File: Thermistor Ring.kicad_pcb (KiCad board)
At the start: 2 copper layers, 70 x 70 mm, 20 parts, among them IC1 MAX30210ENL+, IC2 MAX30210ENL+, IC3 MAX30210ENL+, IC4 MAX30210ENL+, IC5 MAX30210ENL+, IC6 MAX30210ENL+, J1 Conn_01x04_Socket, J3 Conn_01x03_Socket, U1 TPS7A2018PDBVR

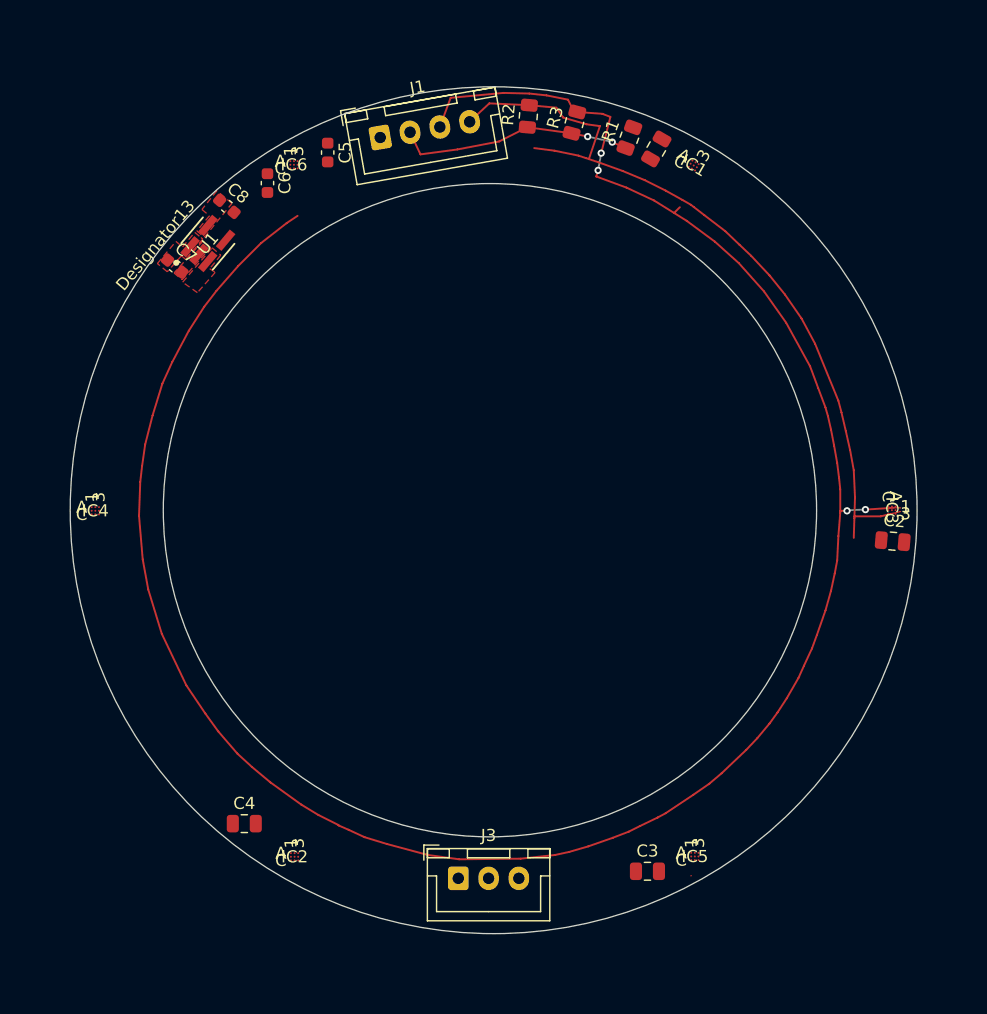
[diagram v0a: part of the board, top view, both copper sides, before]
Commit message: v0.1 alpha for review
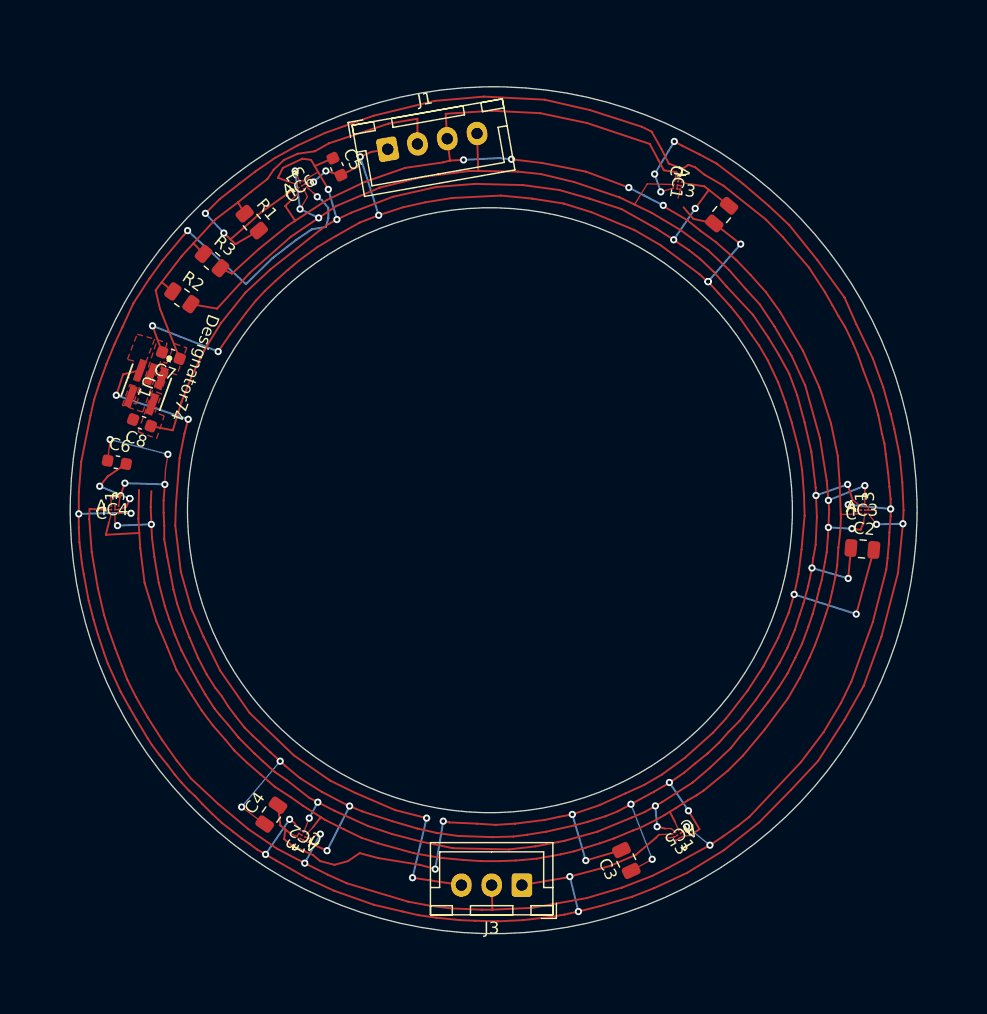
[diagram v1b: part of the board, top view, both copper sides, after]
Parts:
- U1: footprint LDO_TSA7A:DBV0005A-IPC_A -> TPS7A201:DBV0005A-IPC_A
- moved R2 32.3 mm to (188.1, 53.6), turned to -35 degrees
- moved R3 32.1 mm to (190.6, 50.5), turned to -40 degrees
- moved R1 32.0 mm to (193.9, 47.3), turned to -50 degrees
- moved C6 26.2 mm to (182.8, 67.2), turned to -10 degrees
- moved C8 19.2 mm to (184.8, 63.9), turned to 160 degrees
- moved U1 12.9 mm to (185.2, 61.0), turned to -110 degrees
- moved C1 7.66 mm to (232.8, 46.7), turned to -130 degrees
- moved C7 7.40 mm to (187.2, 58.3), turned to 160 degrees
- moved J3 5.28 mm to (216.3, 102.1), turned to 180 degrees
- moved C2 2.59 mm to (244.4, 74.3)
- moved C4 2.36 mm to (195.5, 96.3), turned to 55 degrees
- moved IC5 2.27 mm to (229.1, 98.0), turned to -150 degrees
- moved IC3 2.24 mm to (244.6, 71.1), turned to 0 degrees
- moved IC1 2.11 mm to (229.1, 44.3), turned to -100 degrees
- moved C3 1.96 mm to (224.9, 100.1), turned to 115 degrees
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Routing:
- net /VDD: track 0.00 -> 244.5 mm, vias 0 -> 20
- net /CVT/PDB: track 0.00 -> 224.6 mm, vias 0 -> 13
- net /INT: track 0.00 -> 213.3 mm, vias 0 -> 8
- net GND: track 0.00 -> 195.9 mm, vias 0 -> 18
- net /SCL: track 64.7 -> 196.8 mm, vias 0 -> 13
- net /ENABLE: track 0.00 -> 61.8 mm, vias 0 -> 4
- net /Power 3.3-5V: track 19.6 -> 38.4 mm, vias 2 -> 0
- net /SDA: track 183.6 -> 202.3 mm
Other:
- outline, holes or cut-outs redrawn

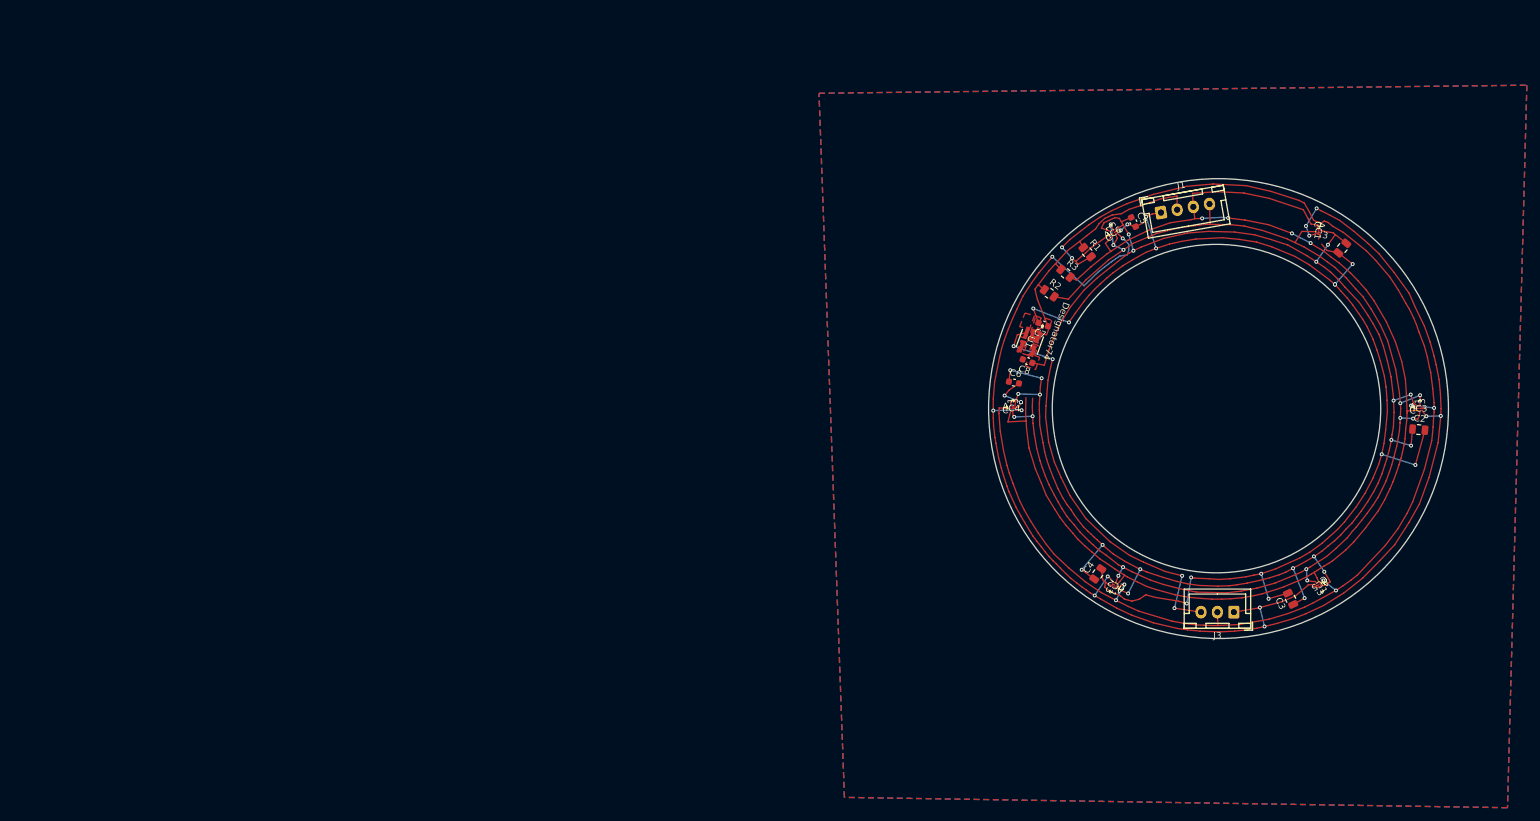
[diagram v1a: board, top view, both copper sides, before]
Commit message: changing to smaller diameter
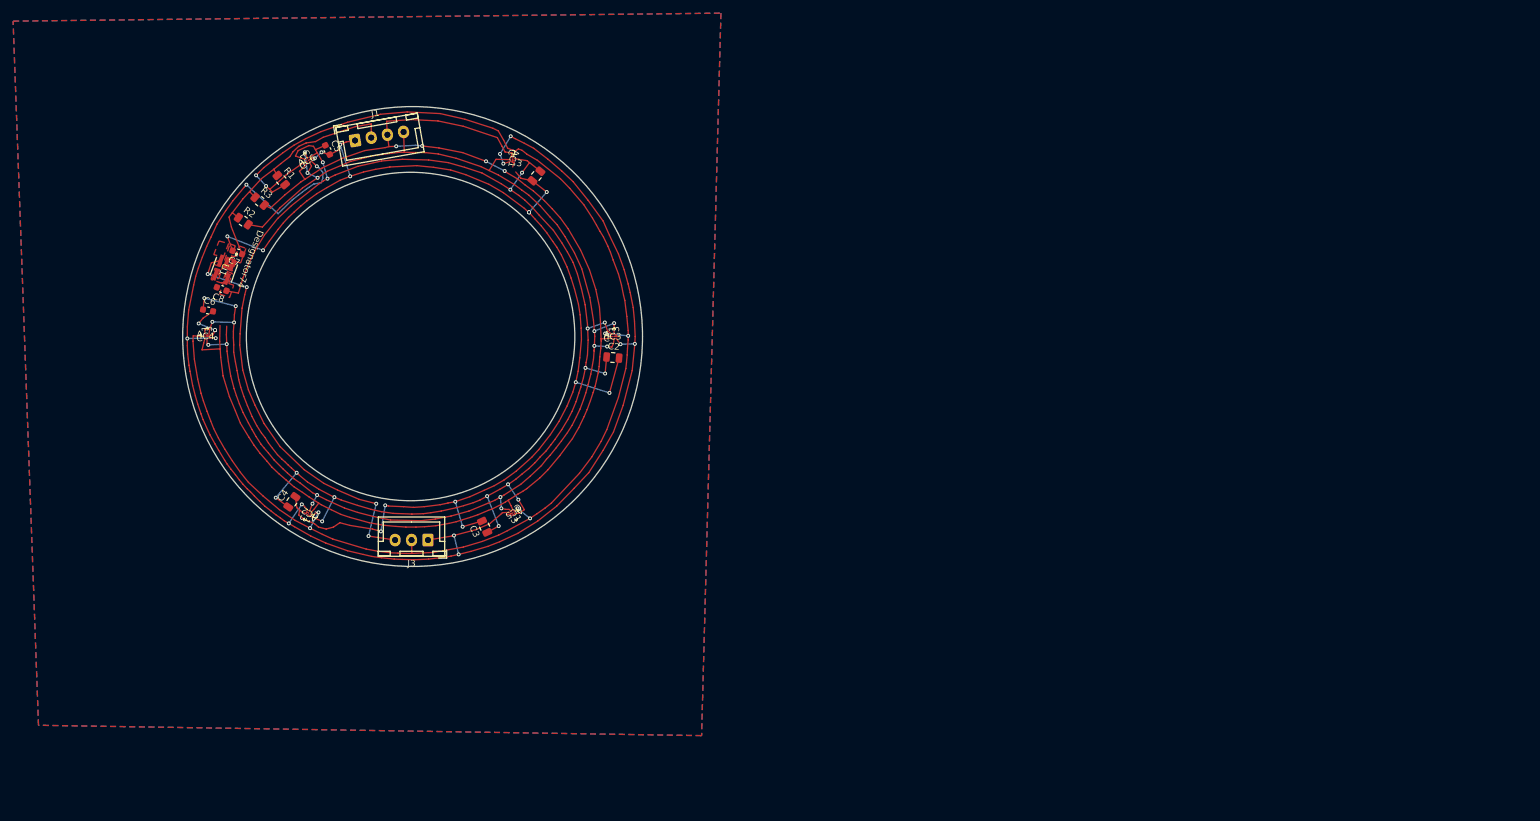
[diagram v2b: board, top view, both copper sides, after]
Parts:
- moved IC2 123.2 mm to (75.4, 87.0)
- moved IC6 123.2 mm to (75.4, 33.3)
- moved J1 123.2 mm to (82.5, 30.3)
- moved R3 123.2 mm to (68.0, 39.6)
- moved C1 123.2 mm to (110.1, 35.7)
- moved C4 123.2 mm to (72.9, 85.3)
- moved C5 123.2 mm to (78.3, 31.8)
- moved C6 123.2 mm to (60.1, 56.2)
- moved IC1 123.2 mm to (106.4, 33.3)
- moved IC5 123.2 mm to (106.4, 87.0)
- moved R1 123.2 mm to (71.2, 36.3)
- moved U1 123.2 mm to (62.5, 50.0)
- moved C2 123.2 mm to (121.7, 63.3)
- moved C3 123.2 mm to (102.2, 89.1)
- moved C7 123.2 mm to (64.6, 47.4)
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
